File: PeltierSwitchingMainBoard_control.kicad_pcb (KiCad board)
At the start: 2 copper layers, 24.6 x 45.1 mm, 24 parts, among them J3 Molex Micro Lock (1.25mm 1.5A), J4 Conn_01x14, U1 HIP4080A

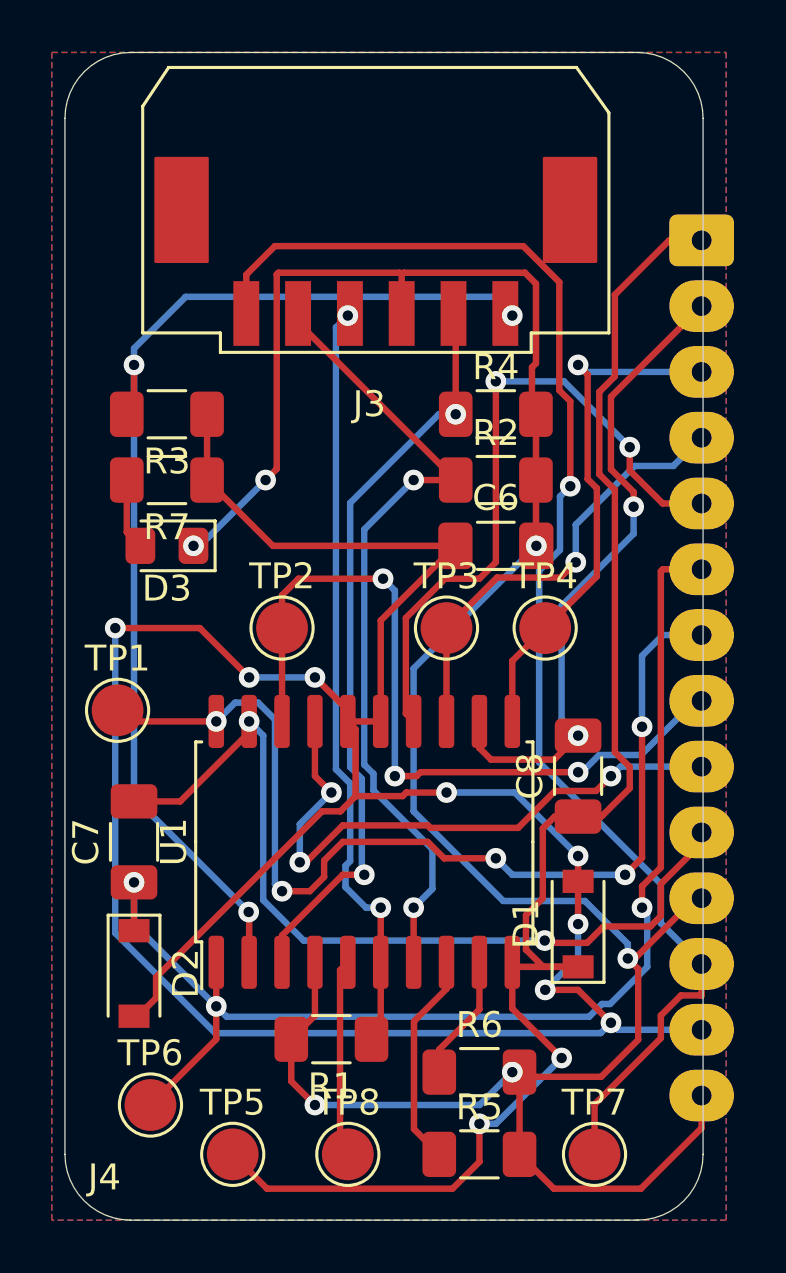
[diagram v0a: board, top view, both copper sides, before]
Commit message: Updated silkscreen
Signed-off-by: bebenlebricolo <benoittarrade@hotmail.fr>
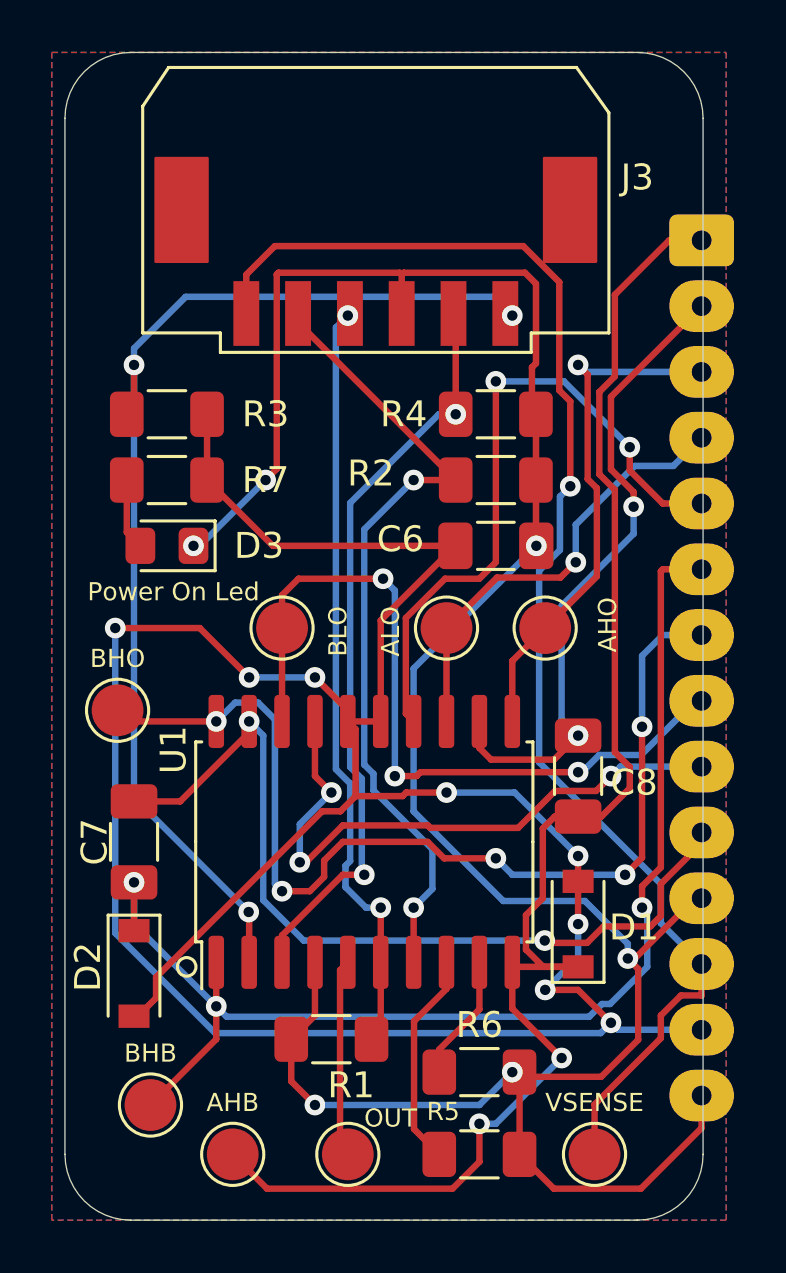
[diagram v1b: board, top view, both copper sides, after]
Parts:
- removed TP8: TestPoint, TestPoint:TestPoint_Pad_D2.0mm
- added OUT: TestPoint, TestPoint:TestPoint_Pad_D2.0mm, F.Cu at (73.0, 79.4)
- renumbered TP5 to AHB, TP4 to AHO, TP3 to ALO, TP6 to BHB, TP1 to BHO, TP2 to BLO, TP7 to VSENSE
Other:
- board text added: "Power On Led"
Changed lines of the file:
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@@
   (general
     (thickness 1.6)
-    (drawings 8)
+    (drawings 10)
     (tracks 359)
     (zones 0)
@@
   (module PeltierSwitchingMainBoard_control:Molex_MicroLock_1.25_01x06 (layer F.Cu)
     (at 78.105 41.91 180)
-    (fp_text reference J3 (at 4.25 -8.5 180) (layer F.SilkS)
+    (fp_text reference J3 (at -6.096 0.254 180) (layer F.SilkS)
       (effects (font (size 1 1) (thickness 0.15)))
     )
@@
   (module PeltierSwitchingMainBoard_control:Mezzanine_board_14contacts locked (layer F.Cu)
     (at 61.684999 82.185)
-    (fp_text reference J4 (at 1.942001 -1.921) (layer F.SilkS)
+    (fp_text reference J4 (at 1.942001 -1.921) (layer F.SilkS) hide
       (effects (font (size 1 1) (thickness 0.15)))
     )
@@
     (tags "SOIC SO")
     (attr smd)
-    (fp_text reference U1 (at 0 -7.35 90) (layer F.SilkS)
+    (fp_text reference U1 (at 3.556 -7.366 90) (layer F.SilkS)
       (effects (font (size 1 1) (thickness 0.15)))
     )
@@
     (tags "test point SMD pad")
     (attr virtual)
-    (fp_text reference TP8 (at 0 -1.998) (layer F.SilkS)
-      (effects (font (size 1 1) (thickness 0.15)))
+    (fp_text reference OUT (at 1.651 -1.397) (layer F.SilkS)
+      (effects (font (size 0.7 0.7) (thickness 0.1)))
     )
     (fp_text value TestPoint (at 0 2.05) (layer F.Fab)
@@
     (tags "test point SMD pad")
     (attr virtual)
-    (fp_text reference TP7 (at 0 -1.998) (layer F.SilkS)
-      (effects (font (size 1 1) (thickness 0.15)))
+    (fp_text reference VSENSE (at 0 -1.998) (layer F.SilkS)
+      (effects (font (size 0.7 0.7) (thickness 0.1)))
     )
     (fp_text value TestPoint (at 0 2.05) (layer F.Fab)
@@
     (tags "test point SMD pad")
     (attr virtual)
-    (fp_text reference TP6 (at 0 -1.998) (layer F.SilkS)
-      (effects (font (size 1 1) (thickness 0.15)))
+    (fp_text reference BHB (at 0 -1.998) (layer F.SilkS)
+      (effects (font (size 0.7 0.7) (thickness 0.1)))
     )
     (fp_text value TestPoint (at 0 2.05) (layer F.Fab)
@@
     (tags "test point SMD pad")
     (attr virtual)
-    (fp_text reference TP5 (at 0 -1.998) (layer F.SilkS)
-      (effects (font (size 1 1) (thickness 0.15)))
+    (fp_text reference AHB (at 0 -1.998) (layer F.SilkS)
+      (effects (font (size 0.7 0.7) (thickness 0.1)))
     )
     (fp_text value TestPoint (at 0 2.05) (layer F.Fab)
@@
     (tags "test point SMD pad")
     (attr virtual)
-    (fp_text reference TP4 (at 0 -1.998) (layer F.SilkS)
-      (effects (font (size 1 1) (thickness 0.15)))
+    (fp_text reference AHO (at 2.413 -0.127 90) (layer F.SilkS)
+      (effects (font (size 0.7 0.7) (thickness 0.1)))
     )
     (fp_text value TestPoint (at 0 2.05) (layer F.Fab)
@@
     (tags "test point SMD pad")
     (attr virtual)
-    (fp_text reference TP3 (at 0 -1.998) (layer F.SilkS)
-      (effects (font (size 1 1) (thickness 0.15)))
+    (fp_text reference ALO (at -2.159 0.127 90) (layer F.SilkS)
+      (effects (font (size 0.7 0.7) (thickness 0.1)))
     )
     (fp_text value TestPoint (at 0 2.05) (layer F.Fab)
@@
     (tags "test point SMD pad")
     (attr virtual)
-    (fp_text reference TP2 (at 0 -1.998) (layer F.SilkS)
-      (effects (font (size 1 1) (thickness 0.15)))
+    (fp_text reference BLO (at 2.159 0.127 90) (layer F.SilkS)
+      (effects (font (size 0.7 0.7) (thickness 0.1)))
     )
     (fp_text value TestPoint (at 0 2.05) (layer F.Fab)
@@
     (tags "test point SMD pad")
     (attr virtual)
-    (fp_text reference TP1 (at 0 -1.998) (layer F.SilkS)
-      (effects (font (size 1 1) (thickness 0.15)))
+    (fp_text reference BHO (at 0 -1.998) (layer F.SilkS)
+      (effects (font (size 0.7 0.7) (thickness 0.1)))
     )
     (fp_text value TestPoint (at 0 2.05) (layer F.Fab)
@@
     (tags "resistor handsolder")
     (attr smd)
-    (fp_text reference R7 (at 0 -1.82) (layer F.SilkS)
+    (fp_text reference R7 (at -3.81 0) (layer F.SilkS)
       (effects (font (size 1 1) (thickness 0.15)))
     )
@@
     (tags "resistor handsolder")
     (attr smd)
-    (fp_text reference R5 (at 0 -1.82) (layer F.SilkS)
-      (effects (font (size 1 1) (thickness 0.15)))
+    (fp_text reference R5 (at -1.397 -1.651) (layer F.SilkS)
+      (effects (font (size 0.7 0.7) (thickness 0.1)))
     )
     (fp_text value 10k (at 0 1.82) (layer F.Fab)
@@
     (tags "resistor handsolder")
     (attr smd)
-    (fp_text reference R4 (at 0 -1.82) (layer F.SilkS)
+    (fp_text reference R4 (at -3.556 0) (layer F.SilkS)
       (effects (font (size 1 1) (thickness 0.15)))
     )
@@
     (tags "resistor handsolder")
     (attr smd)
-    (fp_text reference R3 (at 0 -1.82) (layer F.SilkS)
+    (fp_text reference R3 (at -3.81 0) (layer F.SilkS)
       (effects (font (size 1 1) (thickness 0.15)))
     )
@@
     (tags "resistor handsolder")
     (attr smd)
-    (fp_text reference R2 (at 0 -1.82) (layer F.SilkS)
+    (fp_text reference R2 (at -4.826 -0.254) (layer F.SilkS)
       (effects (font (size 1 1) (thickness 0.15)))
     )
@@
     (tags "resistor handsolder")
     (attr smd)
-    (fp_text reference R1 (at 0 -1.82) (layer F.SilkS)
+    (fp_text reference R1 (at -0.762 -1.778) (layer F.SilkS)
       (effects (font (size 1 1) (thickness 0.15)))
     )
@@
     (tags "LED handsolder")
     (attr smd)
-    (fp_text reference D3 (at 0 -1.65) (layer F.SilkS)
+    (fp_text reference D3 (at -3.556 0) (layer F.SilkS)
       (effects (font (size 1 1) (thickness 0.15)))
     )
@@
     (tags SOD-123)
     (attr smd)
-    (fp_text reference D2 (at 0 -2 90) (layer F.SilkS)
+    (fp_text reference D2 (at -0.254 1.778 270) (layer F.SilkS)
       (effects (font (size 1 1) (thickness 0.15)))
     )
@@
     (tags SOD-123)
     (attr smd)
-    (fp_text reference D1 (at 0 -2 90) (layer F.SilkS)
+    (fp_text reference D1 (at -0.127 2.159 180) (layer F.SilkS)
       (effects (font (size 1 1) (thickness 0.15)))
     )
@@
     (tags "capacitor handsolder")
     (attr smd)
-    (fp_text reference C8 (at 0 -1.85 90) (layer F.SilkS)
+    (fp_text reference C8 (at -0.254 2.159 180) (layer F.SilkS)
       (effects (font (size 1 1) (thickness 0.15)))
     )
@@
     (tags "capacitor handsolder")
     (attr smd)
-    (fp_text reference C7 (at 0 -1.85 90) (layer F.SilkS)
+    (fp_text reference C7 (at 0 -1.524 90) (layer F.SilkS)
       (effects (font (size 1 1) (thickness 0.15)))
     )
@@
     (tags "capacitor handsolder")
     (attr smd)
-    (fp_text reference C6 (at 0 -1.85) (layer F.SilkS)
+    (fp_text reference C6 (at -3.683 -0.254) (layer F.SilkS)
       (effects (font (size 1 1) (thickness 0.15)))
     )
@@
     )
   )
+  (gr_circle (center 66.802 72.136) (end 67.056 72.39) (layer F.SilkS) (width 0.12))
+  (gr_text "Power On Led" (at 66.294 57.658) (layer F.SilkS)
+    (effects (font (size 0.7 0.7) (thickness 0.1)))
+  )
   (gr_line (start 64.643 81.915) (end 84.201 81.915) (layer Edge.Cuts) (width 0.05))
